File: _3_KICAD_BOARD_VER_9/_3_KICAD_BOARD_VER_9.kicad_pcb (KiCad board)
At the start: 4 copper layers, 163.6 x 87 mm, 60 parts, among them J1 HTEC8-160-01-X-DV-A-BL-X, J2 PH2-20-UA, J3 PH2-20-UA, J4 PH2-20-UA, J5 PH2-20-UA, J6 PH2-20-UA, U1 AZ1117H-3.3TRE1, U2 dsPIC33AK512MPS505T-I/PT, U3 DAC7564ICPW, U4 FM24W256G, Y1 ABMM-25.000MHZ-B2-T

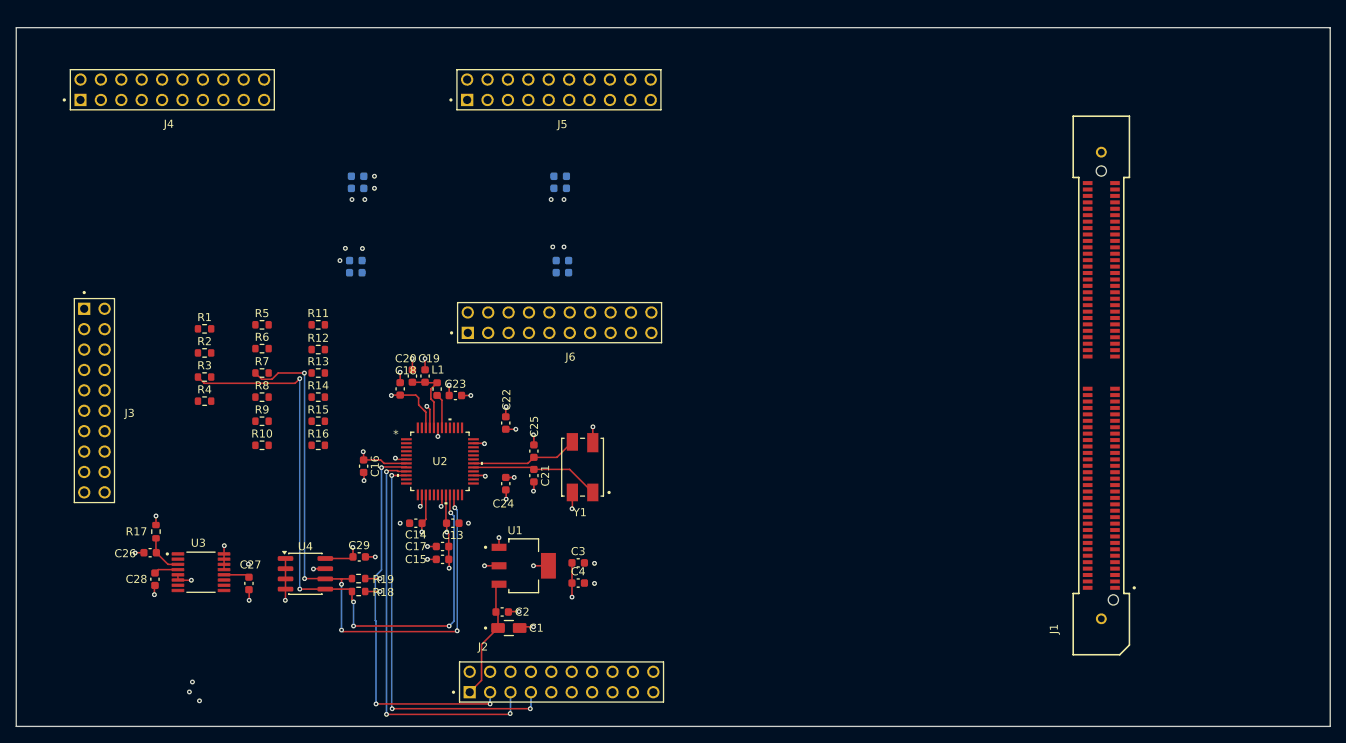
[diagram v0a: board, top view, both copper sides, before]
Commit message: feat : dim only project done
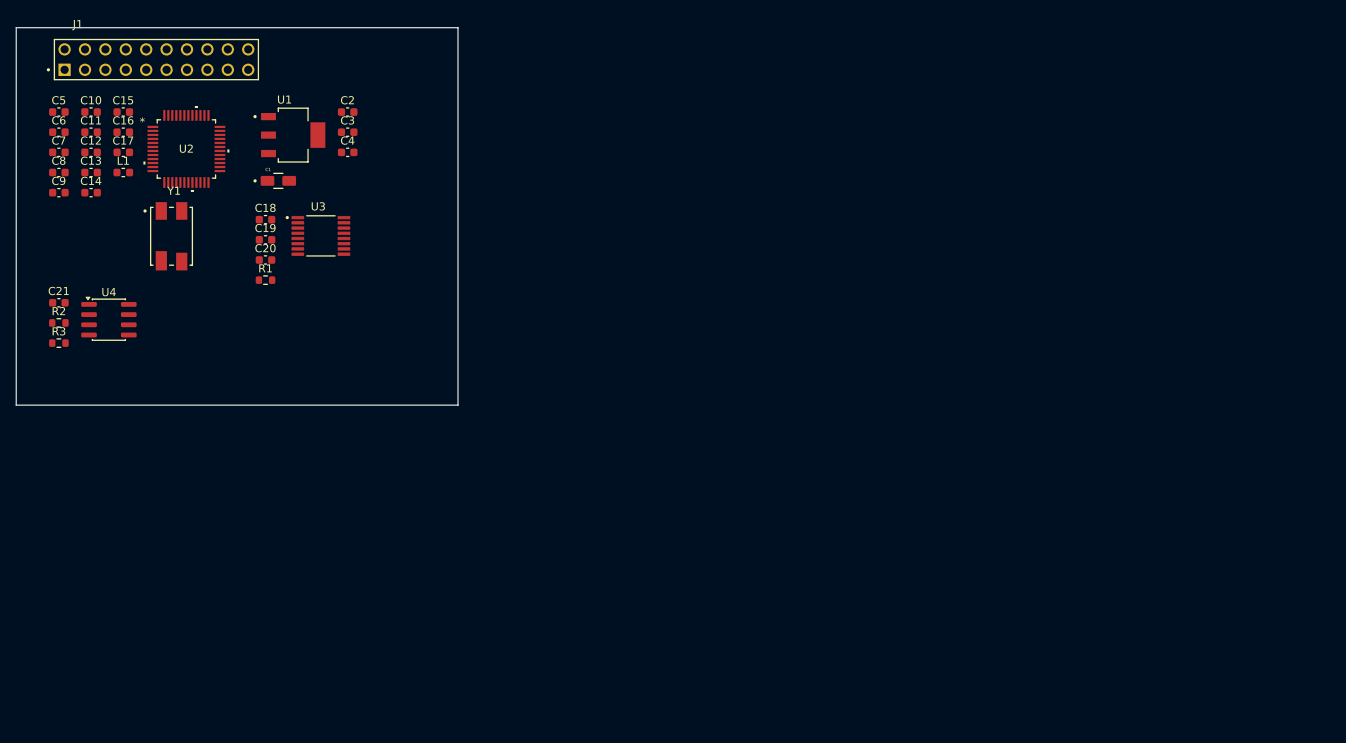
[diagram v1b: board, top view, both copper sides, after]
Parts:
- removed C22, C23, C24, C26, C27, C28, C29: 100nF, Capacitor_SMD:C_0603_1608Metric
- removed C25: 18pF, Capacitor_SMD:C_0603_1608Metric
- removed J2, J3, J4, J5, J6: PH2-20-UA, PH2-20-UA:ADAM_PH2-20-UA
- removed R10, R11, R12, R13, R14, R15, R16, R4, R5, R6, R7, R8, R9: 0R, Resistor_SMD:R_0603_1608Metric
- removed R17: 100R, Resistor_SMD:R_0603_1608Metric
- removed R18, R19: 2.2K, Resistor_SMD:R_0603_1608Metric
- C10, C6: moved to F.Cu
- C11: value 100nF -> 10uF; moved to F.Cu
- C12, C5, C8: value 22uF -> 100nF; moved to F.Cu
- C13: value 100nF -> 18pF
- C15: value 47uF -> 100nF
- C17: value 1uF -> 18pF
- C19: value 10uF -> 100nF
- C21: value 18pF -> 100nF
- C7: value 100nF -> 47uF; moved to F.Cu
- C9: value 22uF -> 1uF; moved to F.Cu
- J1: value HTEC8-160-01-X-DV-A-BL-X -> PH2-20-UA; footprint HTEC8-160-01-X-DV-A-BL-X:SAMTEC_HTEC8-160-01-X-DV-A-BL-X -> PH2-20-UA:ADAM_PH2-20-UA
- R1: value 0R -> 100R
- R2, R3: value 0R -> 2.2K
- moved J1 124.5 mm to (102.5, 57.0), turned to 0 degrees
- moved C15 68.4 mm to (98.3, 63.5), turned to 0 degrees
- moved C2 65.1 mm to (126.3, 63.5)
- moved C17 63.2 mm to (98.3, 68.5), turned to 0 degrees
- moved C21 62.9 mm to (90.3, 87.3), turned to 0 degrees
- moved C13 62.7 mm to (94.3, 71.0)
- moved C1 62.6 mm to (117.6, 72.1)
- moved C9 62.4 mm to (90.3, 73.5)
- moved C11 61.2 mm to (94.3, 66.0)
- moved C3 60.8 mm to (126.3, 66.0)
- moved C4 60.8 mm to (126.3, 68.5)
- moved U1 60.8 mm to (119.5, 66.4)
- moved C12 60.2 mm to (94.3, 68.5)
- moved C10 59.0 mm to (94.3, 63.5)
- moved Y1 58.7 mm to (104.3, 79.0), turned to 0 degrees
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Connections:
- net /DIM_SHEET/SPI_BUS.MOSI renamed /MCU_48PIN_SHEET/SPI_BUS.MOSI
- net /DIM_SHEET/SPI_BUS.SCLK renamed /MCU_48PIN_SHEET/SPI_BUS.SCLK
- net /DIM_SHEET/SPI_BUS.SS renamed /MCU_48PIN_SHEET/SPI_BUS.SS
- C11 pad 1: +3.3V -> /MCU_48PIN_SHEET/VDD_CORE
- C12 pad 1: +3.3V -> /MCU_48PIN_SHEET/VDD_CORE
- C13 pad 1: +3.3V -> Net-(U2-OSCO/CLKO/RP33/IOMAF5/RC0)
- C17 pad 1: +3.3V -> Net-(U2-OSCI/CLKI/RP34/IOMAF6/RC1)
- C18 pad 1: +3.3V -> Net-(U3-VREFH/VREFOUT)
- C19 pad 1: /MCU_48PIN_SHEET/VDD_CORE -> +3.3V
- C20 pad 1: /MCU_48PIN_SHEET/VDD_CORE -> +3.3V
- C21 pad 1: Net-(U2-OSCO/CLKO/RP33/IOMAF5/RC0) -> +3.3V
- J1 pad 1: /DIM_SHEET/DIM_BUS.IO0 -> VIN
- J1 pad 10: unconnected-(J1-Pad10) -> /MCU_48PIN_SHEET/DEBUG_BUS.PGD
- J1 pad 11: /DIM_SHEET/DIM_BUS.IO6 -> /MCU_48PIN_SHEET/ADC_BUS._B1
- J1 pad 12: Net-(J1-Pad12) -> /MCU_48PIN_SHEET/DEBUG_BUS.PGC
- J1 pad 13: /DIM_SHEET/DIM_BUS.IO8 -> /MCU_48PIN_SHEET/ADC_BUS._B2
- J1 pad 14: Net-(J1-Pad14) -> /MCU_48PIN_SHEET/DEBUG_BUS.MCLR
- J1 pad 15: /DIM_SHEET/DIM_BUS.IO10 -> /SIGNAL_IO_SHEET/DAC_BUS._0
- J1 pad 16: /DIM_SHEET/DIM_BUS.IO7 -> +3.3V
- J1 pad 17: unconnected-(J1-Pad17) -> /SIGNAL_IO_SHEET/DAC_BUS._1
- J1 pad 18: /DIM_SHEET/DIM_BUS.IO9 -> /MCU_48PIN_SHEET/SYS_BUS.BAND_SELECT
- J1 pad 19: unconnected-(J1-Pad19) -> /SIGNAL_IO_SHEET/DAC_BUS._2
- J1 pad 2: /DIM_SHEET/DIM_BUS.IO1 -> +3.3V
- J1 pad 20: /DIM_SHEET/DIM_BUS.IO11 -> GND
- J1 pad 3: /DIM_SHEET/DIM_BUS.IO2 -> /MCU_48PIN_SHEET/ADC_BUS._A0
- J1 pad 4: /DIM_SHEET/DIM_BUS.IO3 -> GND
- J1 pad 5: Net-(J1-Pad5) -> /MCU_48PIN_SHEET/ADC_BUS._A1
- J1 pad 6: /DIM_SHEET/DIM_BUS.IO5 -> /MCU_48PIN_SHEET/UART_BUS.TX
- J1 pad 7: Net-(J1-Pad7) -> /MCU_48PIN_SHEET/ADC_BUS._A2
- J1 pad 8: unconnected-(J1-Pad8) -> /MCU_48PIN_SHEET/UART_BUS.RX
- J1 pad 9: /DIM_SHEET/DIM_BUS.IO4 -> /MCU_48PIN_SHEET/ADC_BUS._B0
- R1 pad 1: /DIM_SHEET/DEBUG_BUS.MCLR -> +3.3V
- R1 pad 2: Net-(J1-Pad47) -> Net-(U3-VREFH/VREFOUT)
- R2 pad 1: /DIM_SHEET/DEBUG_BUS.PGC -> /MCU_48PIN_SHEET/I2C_BUS.SDA
- R2 pad 2: Net-(J1-Pad51) -> +3.3V
- R3 pad 1: /DIM_SHEET/I2C_BUS.SDA -> /MCU_48PIN_SHEET/I2C_BUS.SCL
- R3 pad 2: Net-(J1-Pad5) -> +3.3V
- U2 pad 10: /DIM_SHEET/ADC_BUS._A2 -> /MCU_48PIN_SHEET/ADC_BUS._A2
- U2 pad 16: /DIM_SHEET/ADC_BUS._B0 -> /MCU_48PIN_SHEET/ADC_BUS._B0
- U2 pad 17: /DIM_SHEET/ADC_BUS._B1 -> /MCU_48PIN_SHEET/ADC_BUS._B1
- U2 pad 18: /DIM_SHEET/ADC_BUS._B2 -> /MCU_48PIN_SHEET/ADC_BUS._B2
- U2 pad 21: /DIM_SHEET/I2C_BUS.SDA -> /MCU_48PIN_SHEET/I2C_BUS.SDA
- U2 pad 22: /DIM_SHEET/I2C_BUS.SCL -> /MCU_48PIN_SHEET/I2C_BUS.SCL
- U2 pad 26: /DIM_SHEET/SPI_BUS.MISO -> /MCU_48PIN_SHEET/SPI_BUS.MISO
- U2 pad 31: /DIM_SHEET/DEBUG_BUS.PGC -> /MCU_48PIN_SHEET/DEBUG_BUS.PGC
- U2 pad 32: /DIM_SHEET/DEBUG_BUS.PGD -> /MCU_48PIN_SHEET/DEBUG_BUS.PGD
- U2 pad 38: /DIM_SHEET/SYS_BUS.BAND_SELECT -> /MCU_48PIN_SHEET/SYS_BUS.BAND_SELECT
- U2 pad 40: /DIM_SHEET/UART_BUS.TX -> /MCU_48PIN_SHEET/UART_BUS.TX
- U2 pad 47: /DIM_SHEET/UART_BUS.RX -> /MCU_48PIN_SHEET/UART_BUS.RX
- U2 pad 48: /DIM_SHEET/DEBUG_BUS.MCLR -> /MCU_48PIN_SHEET/DEBUG_BUS.MCLR
- U2 pad 8: /DIM_SHEET/ADC_BUS._A0 -> /MCU_48PIN_SHEET/ADC_BUS._A0
- U2 pad 9: /DIM_SHEET/ADC_BUS._A1 -> /MCU_48PIN_SHEET/ADC_BUS._A1
- U4 pad 5: /DIM_SHEET/I2C_BUS.SDA -> /MCU_48PIN_SHEET/I2C_BUS.SDA
- U4 pad 6: /DIM_SHEET/I2C_BUS.SCL -> /MCU_48PIN_SHEET/I2C_BUS.SCL
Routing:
- net /DIM_SHEET/I2C_BUS.SDA: track 79.1 -> 0.00 mm, vias 6 -> 0
- net /DIM_SHEET/I2C_BUS.SCL: track 76.3 -> 0.00 mm, vias 6 -> 0
- net +3.3V: track 55.9 -> 0.00 mm, vias 21 -> 0
- net /DIM_SHEET/ADC_BUS._A1: track 50.9 -> 0.00 mm, vias 3 -> 0
- net /DIM_SHEET/ADC_BUS._A2: track 50.3 -> 0.00 mm, vias 3 -> 0
- net GND: track 49.8 -> 0.00 mm, vias 41 -> 0
- net /DIM_SHEET/ADC_BUS._A0: track 48.6 -> 0.00 mm, vias 3 -> 0
- net Net-(U2-OSCO/CLKO/RP33/IOMAF5/RC0): track 16.2 -> 0.00 mm
- net VIN: track 15.2 -> 0.00 mm
- net Net-(U2-OSCI/CLKI/RP34/IOMAF6/RC1): track 13.4 -> 0.00 mm
- net /MCU_48PIN_SHEET/VDD_CORE: track 9.19 -> 0.00 mm
- net Net-(U3-VREFH/VREFOUT): track 5.11 -> 0.00 mm
- net /MCU_48PIN_SHEET/LX: track 4.29 -> 0.00 mm
- net /SIGNAL_IO_SHEET/DAC_BUS._2: vias 1 -> 0
- net /SIGNAL_IO_SHEET/DAC_BUS._1: vias 1 -> 0
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- removed copper zone on In2.Cu, net +3.3V
- removed copper zone on In1.Cu, net GND
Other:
- board size 163.6 x 87 mm -> 55 x 47 mm
- copper layers 4 -> 2
